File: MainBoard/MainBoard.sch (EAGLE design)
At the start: 83 parts, among them CN9 UX60SC-MB-5ST, J1 53375-0610, J2 53375-0610, J3 53375-0610, J4 53375-0610, J5 53375-0610, J6 53375-0610, U1 MCP1700T-33, U2 ADR5041, U3 FT232RL, U4 LM5160QPWPRQ1, U5 LPC1549JBD48

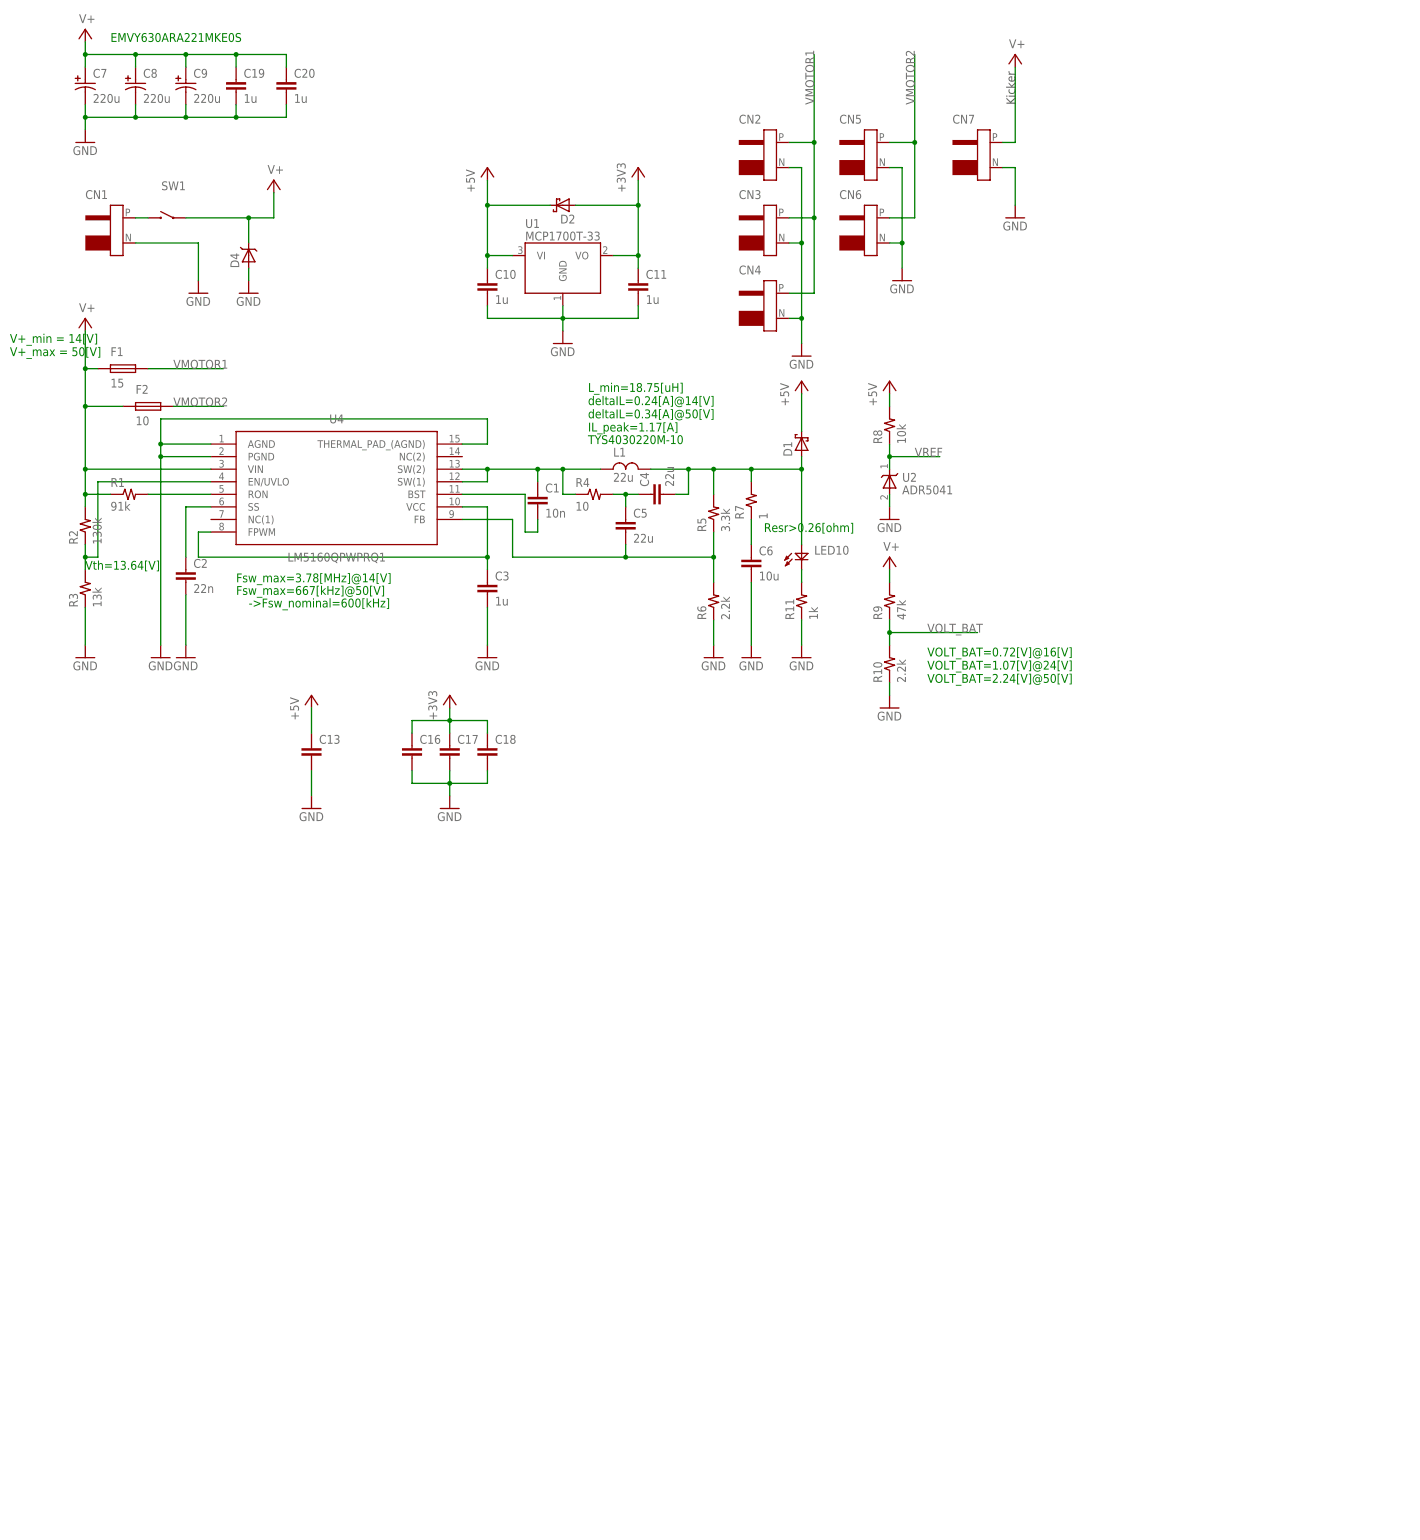
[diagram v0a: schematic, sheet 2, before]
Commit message: tmpからもってきた
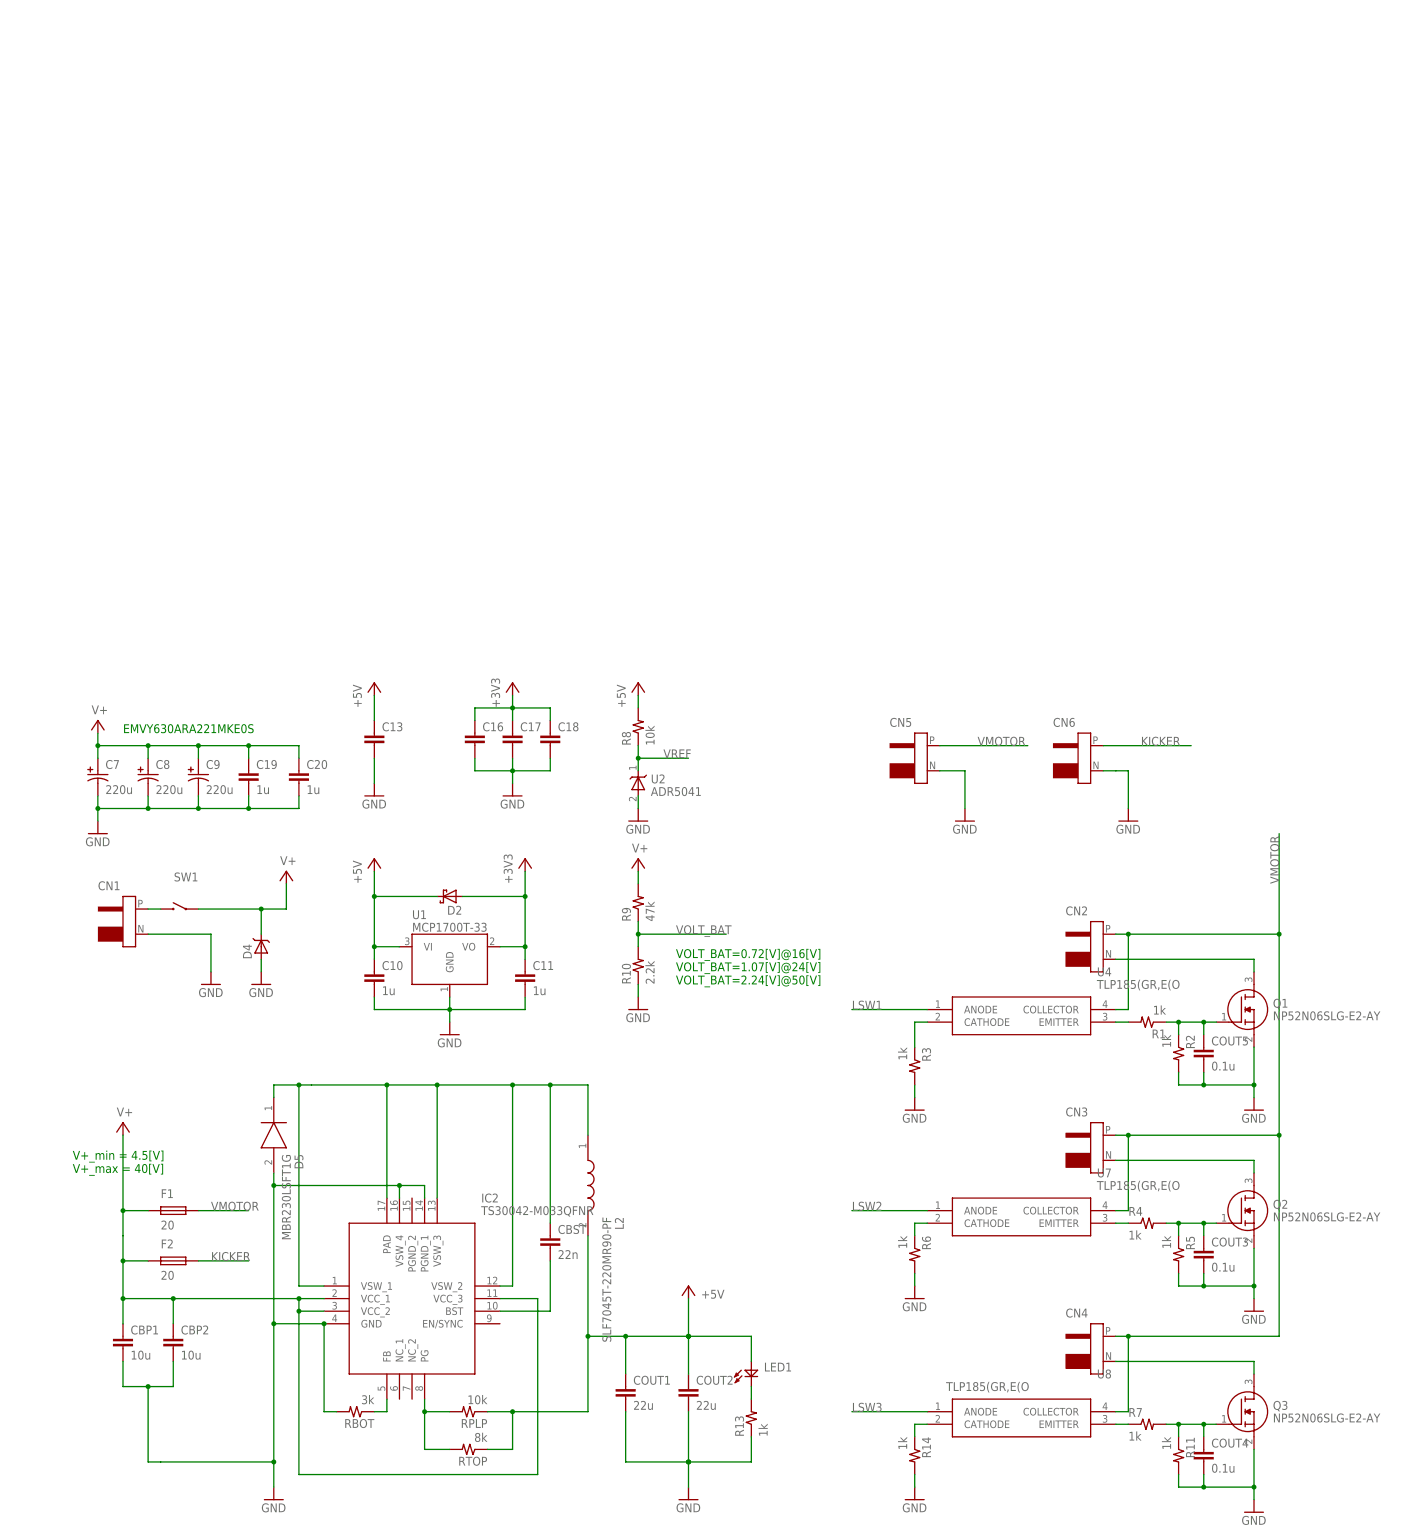
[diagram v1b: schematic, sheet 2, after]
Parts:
- removed C15: 0.1u, MotorDriver:C1608
- removed C4, C5: 22u, MotorDriver:C1608
- removed C6: 10u, MotorDriver:C1608
- removed CN7: (no value), Connector:T-CON
- removed CN9: UX60SC-MB-5ST, con-Hirose:UX60SC-MB-5ST
- removed D1: (no value), MotorDriver:SBD-DO-214AC
- removed L1: 22u, Passive:L40
- removed LED10, LED2, LED3, LED4, LED5, LED6, LED7, LED8: (no value), MotorDriver:LED1608
- removed R17, R18, R19, R20: 220, MotorDriver:R1608
- removed R21: (no value), MotorDriver:R1608
- removed SW2: (no value), MotorDriver:SKRP
- removed U3: FT232RL, ic-FTDI:FT232RL
- added CBP1, CBP2: 10u, MotorDriver:C1608
- added CBST: 22n, MotorDriver:C1608
- added COUT1, COUT2: 22u, MotorDriver:C1608
- added COUT3, COUT4, COUT5: 0.1u, MotorDriver:C1608
- added D5: MBR230LSFT1G, MBR230LSFT1G:MBR230LSFT1G
- added GND: UX60SC-MB-5ST, con-Hirose:UX60SC-MB-5ST
- added IC1: ESP-WROOM-02, esp-wroom-02:ESP-WROOM-02
- added IC2: TS30042-M033QFNR, TS30042-M033QFNR:TS30042-M033QFNR
- added IC3: MAX33053EASA+, MAX33053EASA+:MAX33053EASA+
- added L2: SLF7045T-220MR90-PF, SLF7045T-220MR90-PF:SLF7045T-220MR90-PF
- added Q1, Q2, Q3: NP52N06SLG-E2-AY, NP52N06SLG-E2-AY:NP52N06SLG-E2-AY
- added RBOT: 3k, MotorDriver:R1608
- added RPLP: 10k, MotorDriver:R1608
- added RTOP: 8k, MotorDriver:R1608
- added U6: ESP-WROOM-32, esp32:ESP-WROOM-32
- added U7, U8: TLP185(GR,E(O, TLP185(GR_E(O:TLP185(GR,E(O
- added Y1: CSTCE12M0G55-R0, CSTCE12M0G55-R0:CSTCE12M0G55-R0
- C1: value 10n -> 0.1u
- C2: value 22n -> 33p
- C3: value 1u -> 33p
- F1: value 15 -> 20
- F2: value 10 -> 20
- J1: value 53375-0610 -> 53375-0310; device MotorDriver:53375-0610 -> 53375-0310:53375-0310; SPICEPREFIX (none) -> X
- J2, J3, J4, J5, J6: value 53375-0610 -> 53375-0310; device MotorDriver:53375-0610 -> 53375-0310:53375-0310
- R1: value 91k -> 1k
- R13, R14: value 220 -> 1k
- R15, R16: value 220 -> 120
- R2: value 130k -> 1k
- R3: value 13k -> 1k
- R4: value 10 -> 1k
- R5: value 3.3k -> 1k
- R6: value 2.2k -> 1k
- R7: value 1 -> 1k
- U4: value LM5160QPWPRQ1 -> TLP185(GR,E(O; device LM5160QPWPRQ1:LM5160QPWPRQ1 -> TLP185(GR_E(O:TLP185(GR,E(O
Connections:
- removed net !CS1: J1.2, U5.PIO0_1/ADC0_7/SCT0_OUT4
- removed net !CS2: J2.2, U5.PIO0_2/ADC0_6/SCT1_OUT3
- removed net !CS3: J3.2, U5.PIO0_5/ADC0_3
- removed net !CS4: J4.2, U5.PIO0_7/ADC0_1
- removed net !CS5: J5.2, U5.PIO0_8/ADC0_0/TDO
- removed net !CS6: J6.2, U5.PIO0_9/ADC1_1/TDI
- removed net !ISP: C15.1, R21.1, SW2.B1, SW2.B2, U5.PIO0_16/ADC1_9, U5.PIO0_4/ADC0_4
- removed net CLK: J1.5, J2.5, J3.5, J4.5, J5.5, J6.5
- removed net LED1: LED1.A, U5.PIO0_13/ADC1_6
- removed net LED2: LED2.A, U5.PIO0_17/WAKEUP/!TRST
- removed net LED3: LED3.A, U5.SWCLK/PIO0_19/TCK
- removed net LED4: LED4.A, U5.SWDIO/PIO0_20/SCT1_OUT6/TMS
- removed net LED5: LED5.A, U5.PIO2_12/USB_DP
- removed net LED6: LED6.A, U5.PIO2_13/USB_DM
- removed net LED7: LED7.A, U5.PIO0_24/SCT0_OUT6
- removed net LED8: LED8.A, U5.PIO0_25/ACMP0_I4
- removed net MISO: J1.3, J2.3, J3.3, J4.3, J5.3, J6.3, U5.PIO0_6/ADC0_2/SCT2_OUT3
- removed net MOSI: J1.4, J2.4, J3.4, J4.4, J5.4, J6.4, U5.PIO0_3/ADC0_5/SCT1_OUT4
- removed net N$11: C4.2, D1.A, L1.2, LED10.A, R5.2, R7.2
- removed net N$12: U3.3V3OUT, U3.VCCIO
- removed net N$14: CN9.D-, U3.DM
- removed net N$15: CN9.D+, U3.DP
- removed net N$20 (its old number): LED3.K, R15.2
- removed net N$29: LED4.K, R16.2
- removed net N$30: LED2.K, R14.2
- removed net N$4: C1.1, L1.1, R4.1, U4.SW(1), U4.SW(2)
- removed net VMOTOR1: CN2.P, CN3.P, CN4.P, F1.2
- removed net VMOTOR2: CN5.P, CN6.P, F2.2
- new net !MCLP: J1.1, J2.1, J3.1, J4.1, J5.1, J6.1, U5.PIO0_1/ADC0_7/SCT0_OUT4
- new net +3.3V: IC3.VL
- new net 3.3V: U5.PIO0_2/ADC0_6/SCT1_OUT3
- new net CAN0_RD: IC3.RXD, U5.PIO0_13/ADC1_6
- new net CAN0_TD: IC3.TXD, U5.PIO0_18/SCT0_OUT5
- new net CANH: IC3.CANH, J1.2, J2.2, J3.2, J4.2, J5.2, J6.2, R15.2, R16.1
- new net CANL: IC3.CANL, J1.3, J2.3, J3.3, J4.3, J5.3, J6.3, R15.1, R16.2
- new net D+: GND.D+, U5.PIO2_12/USB_DP
- new net D-: GND.D-, U5.PIO2_13/USB_DM
- new net KICKER: CN6.P, F2.2
- new net LSW1: U4.ANODE, U5.PIO0_6/ADC0_2/SCT2_OUT3
- new net LSW2: U5.PIO0_7/ADC0_1, U7.ANODE
- new net LSW3: U5.PIO0_8/ADC0_0/TDO, U8.ANODE
- new net N$16: CBST.1, D5.K, IC2.PAD, IC2.VSW_1, IC2.VSW_2, IC2.VSW_3, L2.1
- new net N$17: C2.1, U5.RTCXOUT, Y1.1
- new net N$22: IC2.PG, RPLP.2, RTOP.2
- new net N$23: C1.1, IC3.VDD
- new net N$25: R14.1, U8.CATHODE
- new net N$28: COUT4.1, Q3.G, R11.1, R7.2
- new net STBY: IC3.S, U5.PIO0_3/ADC0_5/SCT1_OUT4
- new net VMOTOR: CN2.P, CN3.P, CN4.P, CN5.P, F1.2, U4.COLLECTOR, U7.COLLECTOR, U8.COLLECTOR
- net +3V3: now also IC1.3V3, U6.3V3; no longer R21.2
- net +5V: now also COUT1.1, COUT2.1, L2.2, LED1.A, RPLP.1, RTOP.1; no longer D1.K, J1.1, J2.1, J3.1, J4.1, J5.1, J6.1
- net GND: now also C1.2, CBP1.2, CBP2.2, COUT1.2, COUT2.2, COUT3.2, COUT4.2, COUT5.2, D5.A, GND.GND, GND.S1, GND.S2, IC1.GND0, IC1.GND1, IC1.GND2, IC1.GND3, IC1.IO0, IC2.GND, IC2.PGND_1, IC2.VSW_4, IC3.GND, Q1.S, Q2.S, Q3.S, R11.2, R14.2, R2.2, R3.2, R5.2, R6.2, RBOT.2, U6.GND, U6.GND@1, U6.GND@15, U6.GND@38, Y1.GND; no longer C15.2, C6.2, CN2.N, CN3.N, CN4.N, CN7.N, CN9.GND, CN9.S1, CN9.S2, J1.6, J2.6, J3.6, J4.6, J5.6, J6.6, R11.1, R14.1, R15.1, R16.1, R17.1, R18.1, R19.1, R20.1, R3.1, R6.1, SW2.A1, SW2.A2, U3.AGND, U3.GND, U3.TEST, U4.AGND, U4.PGND, U4.THERMAL_PAD_(AGND)
- net N$1: now also CN2.N, Q1.D; no longer R1.2, U4.RON
- net N$13: now also GND.VBUS; no longer CN9.VBUS, U3.VCC
- net N$19: now also COUT3.1, Q2.G, R4.2, R5.1; no longer LED10.K, R11.2
- net N$2: now also R1.2, U4.EMITTER; no longer R2.1, R3.2, U4.EN/UVLO
- net N$21: now also IC2.FB, RBOT.1; no longer LED5.K, R17.2
- net N$24: now also CBST.2, IC2.BST; no longer LED6.K, R18.2
- net N$26: now also R7.1, U8.EMITTER; no longer LED7.K, R19.2
- net N$27: now also C3.1, U5.RTCXIN, Y1.3; no longer LED8.K, R20.2
- net N$3: now also COUT5.1, Q1.G, R1.1, R2.1; no longer C6.1, R7.1
- net N$5: now also CN3.N, Q2.D; no longer C1.2, U4.BST
- net N$6: now also R3.1, U4.CATHODE; no longer C3.1, U4.FPWM, U4.VCC
- net N$7: now also R6.1, U7.CATHODE; no longer C2.1, U4.SS
- net N$8: now also R4.1, U7.EMITTER; no longer C5.2, R5.1, R6.2, U4.FB
- net N$9: now also CN4.N, Q3.D; no longer C4.1, C5.1, R4.2
- net RX: no longer U3.TXD
- net TX: no longer U3.RXD
- net V+: now also CBP1.1, CBP2.1, IC2.VCC_1, IC2.VCC_2, IC2.VCC_3; no longer CN7.P, R1.1, R2.2, U4.VIN
- net XBEE_RX: now also IC1.RXD, U6.TXD0
- net XBEE_TX: now also IC1.TXD, U6.RXD0
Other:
- note added: "V+_min = 4.5[V] V+_max = 40[V]"
- note removed: "->Fsw_nominal=600[kHz]"
- note removed: "Fsw_max=3.78[MHz]@14[V]"
- note removed: "Fsw_max=667[kHz]@50[V]"
- note removed: "Kicker"
- note removed: "L_min=18.75[uH] deltaIL=0.24[A]@14[V] deltaIL=0.34[A]@50[V] IL_peak=1.17[A]"
- note removed: "Resr>0.26[ohm]"
- note removed: "TYS4030220M-10"
- note removed: "V+_min = 14[V] V+_max = 50[V]"
- note removed: "Vth=13.64[V]"
- moved on the sheet: C10, C11, C12, C13, C14, C16, C17, C18, C19, C20, C7, C8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
